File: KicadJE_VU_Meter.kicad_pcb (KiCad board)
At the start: 2 copper layers, 40 x 128 mm, 62 parts, among them J1 Out, J2 In1, J3 In2, J4 Out, P1 HEADER_2x5_Doepfer, U1 TL072

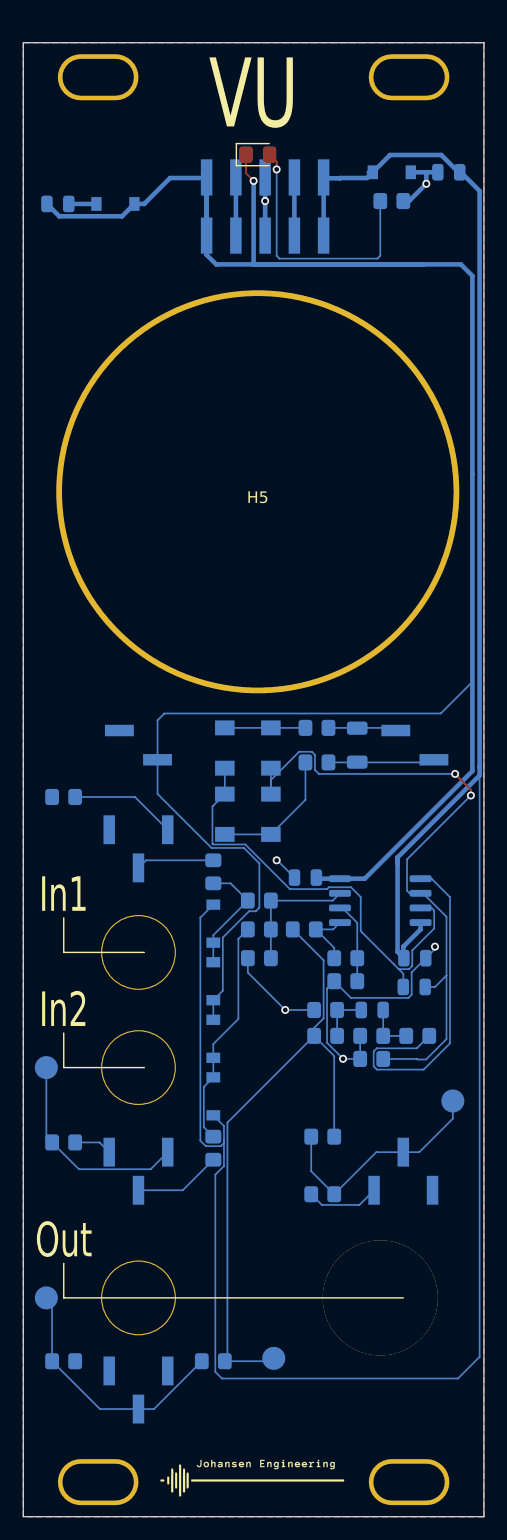
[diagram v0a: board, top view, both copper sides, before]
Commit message: Gerber
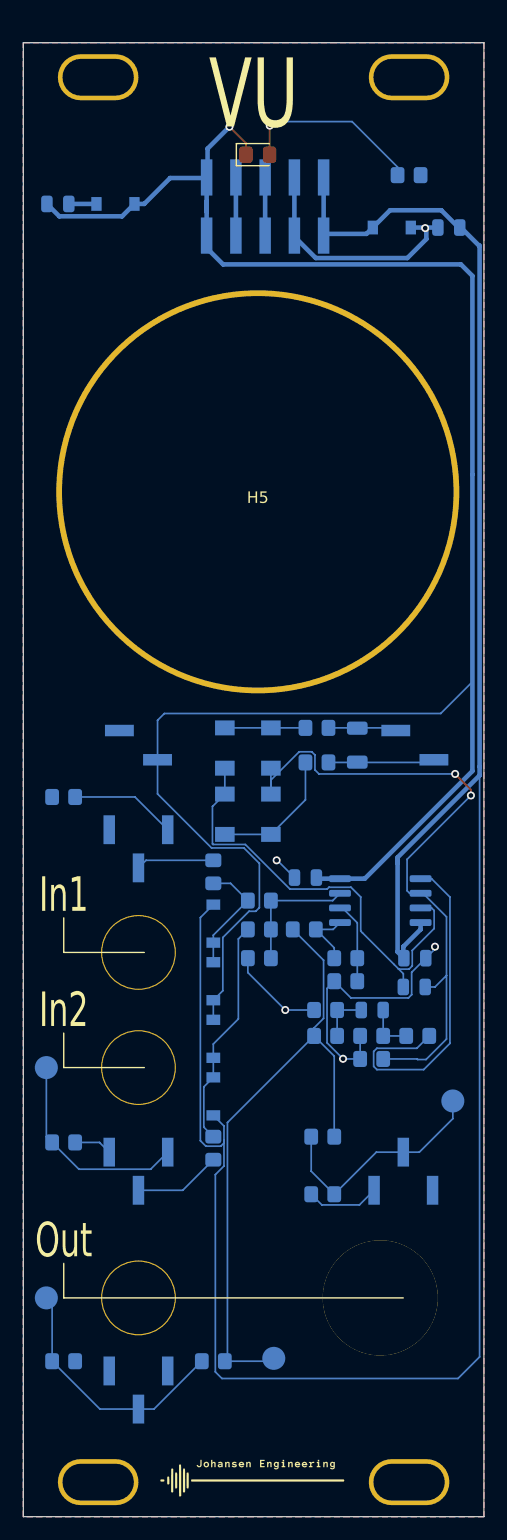
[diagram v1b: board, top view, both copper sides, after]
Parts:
- moved C1 4.80 mm to (136.9, 52.0)
- moved D1 4.80 mm to (132.0, 52.0)
- moved R1 2.70 mm to (133.5, 47.5)
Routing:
- net -12VA: track 217.6 -> 195.5 mm
- net GND: track 67.6 -> 77.8 mm, vias 6 -> 5
- net Net-(D3-Pad2): track 22.7 -> 16.1 mm
- net +12VA: track 217.0 -> 211.7 mm
